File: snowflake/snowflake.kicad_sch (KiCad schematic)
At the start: 19 parts, among them SW1 SK-12E12-G040, U1 RGB, U2 RGB, U25 TPS61022, U3 RGB, U4 RGB

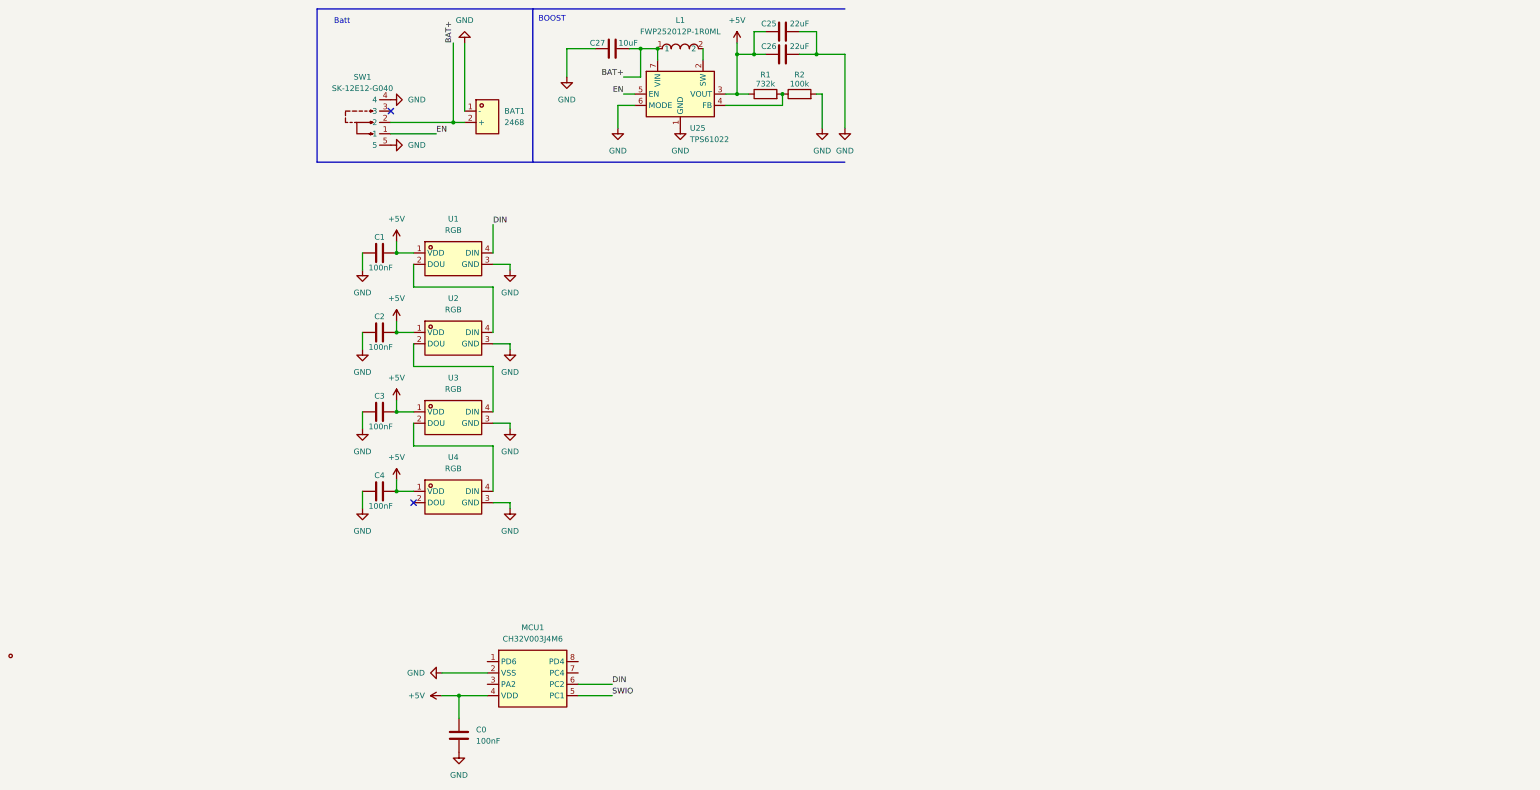
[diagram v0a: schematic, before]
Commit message: 2/6 branches
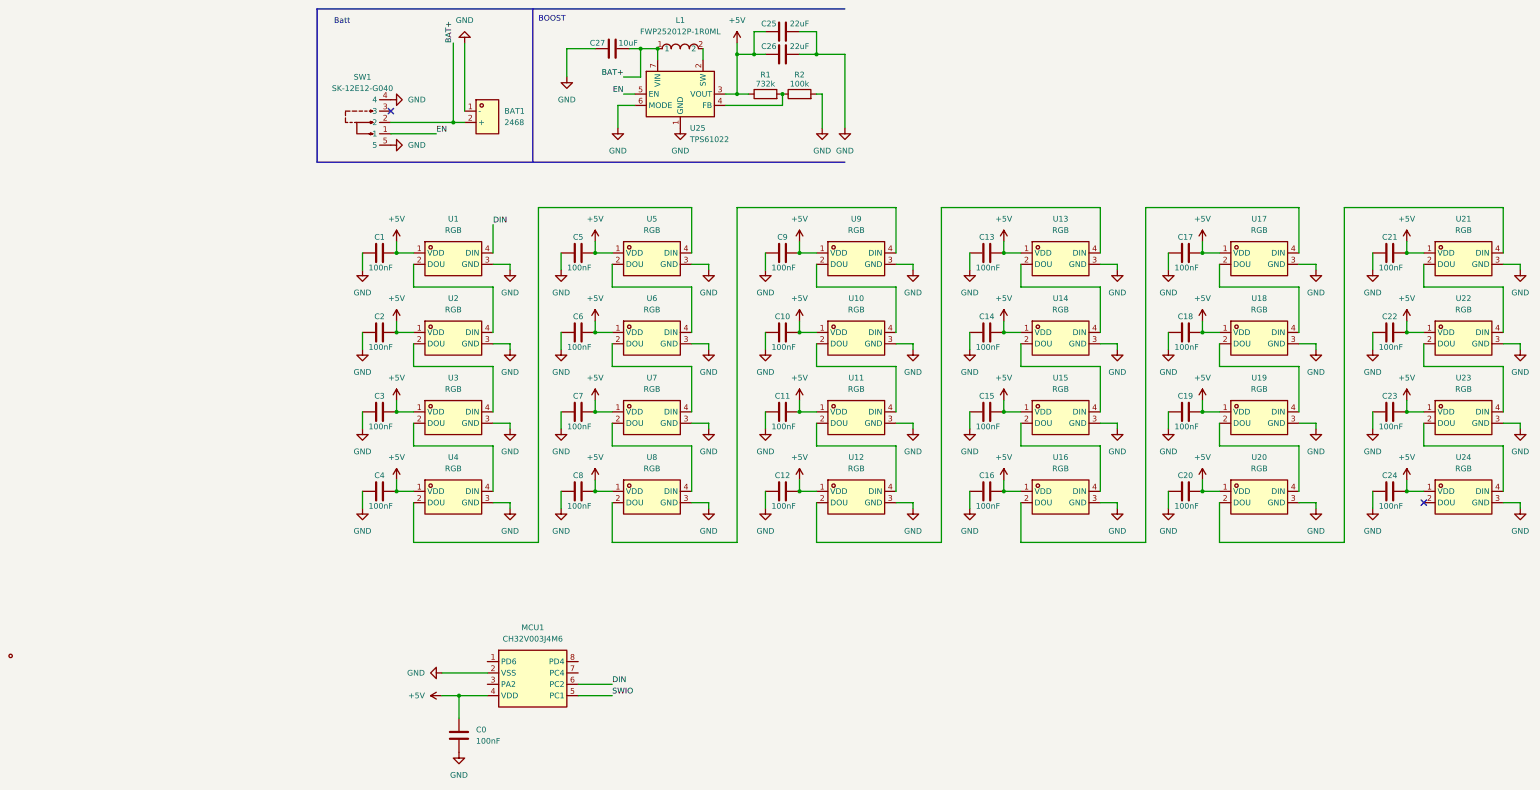
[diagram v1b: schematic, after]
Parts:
- added C10, C11, C12, C13, C14, C15, C16, C17, C18, C19, C20, C21, C22, C23, C24, C5, C6, C7, C8, C9: 100nF, C_0603_1608Metric, symbol Device:C
- added U10, U11, U12, U13, U14, U15, U16, U17, U18, U19, U20, U21, U22, U23, U24, U5, U6, U7, U8, U9: RGB, easyeda2kicad:LED-SMD_4P-L5.0-W5.0-TL_WS2812B-B, symbol easyeda2kicad:TZ-5050S2RGB-5V-I4-H1
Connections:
- net +5V: now also C10.2, C11.2, C12.2, C13.2, C14.2, C15.2, C16.2, C17.2, C18.2, C19.2, C20.2, C21.2, C22.2, C23.2, C24.2, C5.2, C6.2, C7.2, C8.2, C9.2, U10.1 (VDD), U11.1 (VDD), U12.1 (VDD), U13.1 (VDD), U14.1 (VDD), U15.1 (VDD), U16.1 (VDD), U17.1 (VDD), U18.1 (VDD), U19.1 (VDD), U20.1 (VDD), U21.1 (VDD), U22.1 (VDD), U23.1 (VDD), U24.1 (VDD), U5.1 (VDD), U6.1 (VDD), U7.1 (VDD), U8.1 (VDD), U9.1 (VDD)
- net GND: now also C10.1, C11.1, C12.1, C13.1, C14.1, C15.1, C16.1, C17.1, C18.1, C19.1, C20.1, C21.1, C22.1, C23.1, C24.1, C5.1, C6.1, C7.1, C8.1, C9.1, U10.3 (GND), U11.3 (GND), U12.3 (GND), U13.3 (GND), U14.3 (GND), U15.3 (GND), U16.3 (GND), U17.3 (GND), U18.3 (GND), U19.3 (GND), U20.3 (GND), U21.3 (GND), U22.3 (GND), U23.3 (GND), U24.3 (GND), U5.3 (GND), U6.3 (GND), U7.3 (GND), U8.3 (GND), U9.3 (GND)
- net at U4.2 (DOU): now also U5.4 (DIN)
- new net: U5.2 (DOU), U6.4 (DIN)
- new net: U15.2 (DOU), U16.4 (DIN)
- new net: U14.2 (DOU), U15.4 (DIN)
- new net: U10.4 (DIN), U9.2 (DOU)
- new net: U8.2 (DOU), U9.4 (DIN)
- new net: U22.2 (DOU), U23.4 (DIN)
- new net: U21.2 (DOU), U22.4 (DIN)
- new net: U11.2 (DOU), U12.4 (DIN)
- new net: U10.2 (DOU), U11.4 (DIN)
- new net: U18.2 (DOU), U19.4 (DIN)
- new net: U17.2 (DOU), U18.4 (DIN)
- new net: U23.2 (DOU), U24.4 (DIN)
- new net: U7.2 (DOU), U8.4 (DIN)
- new net: U16.2 (DOU), U17.4 (DIN)
- new net: U13.2 (DOU), U14.4 (DIN)
- new net: U12.2 (DOU), U13.4 (DIN)
- new net: U19.2 (DOU), U20.4 (DIN)
- new net: U6.2 (DOU), U7.4 (DIN)
- new net: U20.2 (DOU), U21.4 (DIN)
